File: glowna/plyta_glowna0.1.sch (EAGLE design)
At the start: 217 parts, among them IC1 4504D, IC2 MAX481CSA, IC3 4504D, IC4 OPA4658UU, Q1 CSM-7X-DU, Q2 N-HEXFET-2D_SOT232-IRLL014N, Q3 N-HEXFET-2D_SOT232-IRLL014N, Q4 N-HEXFET-2D_SOT232-IRLL014N, Q5 N-HEXFET-2D_SOT232-IRLL014N, Q6 N-HEXFET-2D_SOT232-IRLL014N, X1 MINI-USB_SHIELD5P2-32005-601

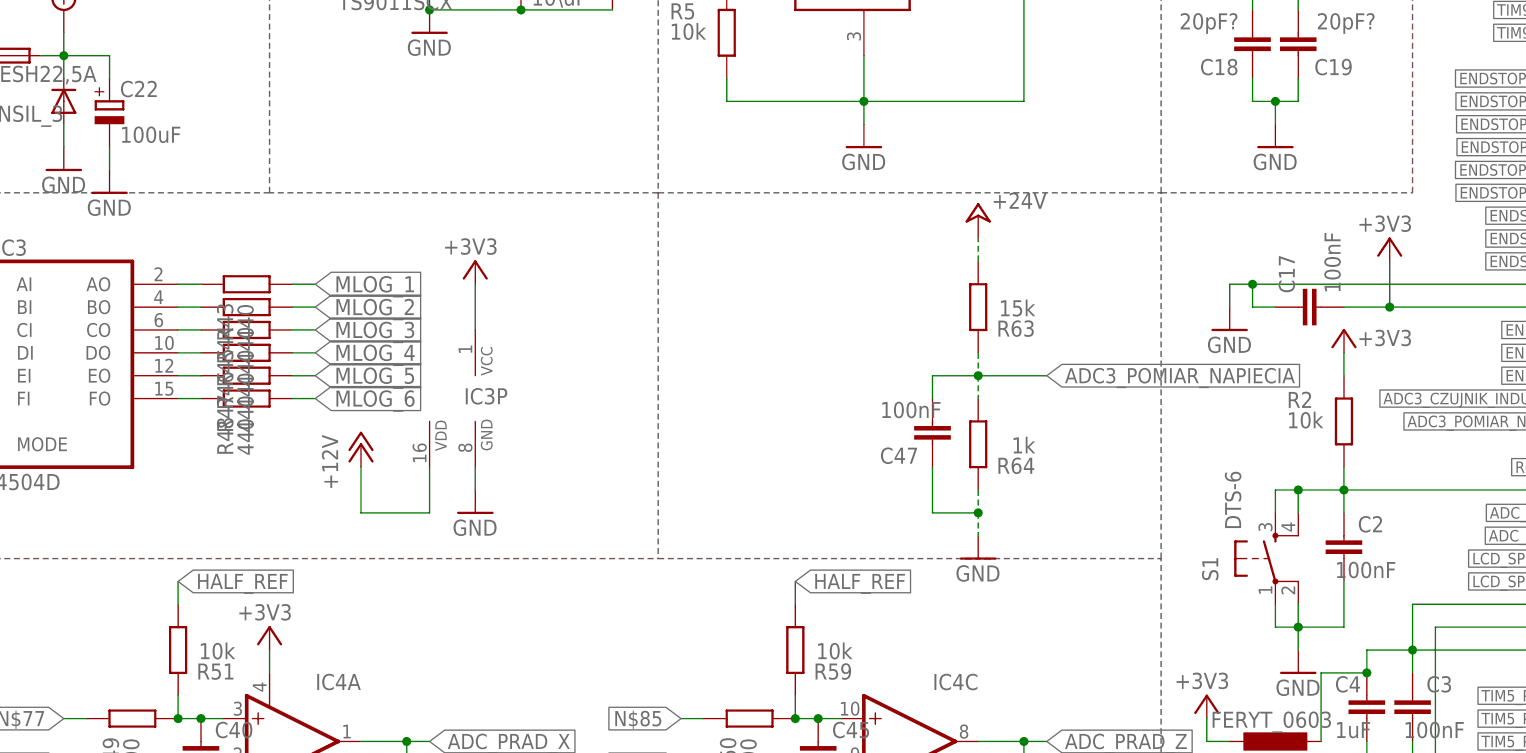
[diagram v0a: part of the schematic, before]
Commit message: zmiana
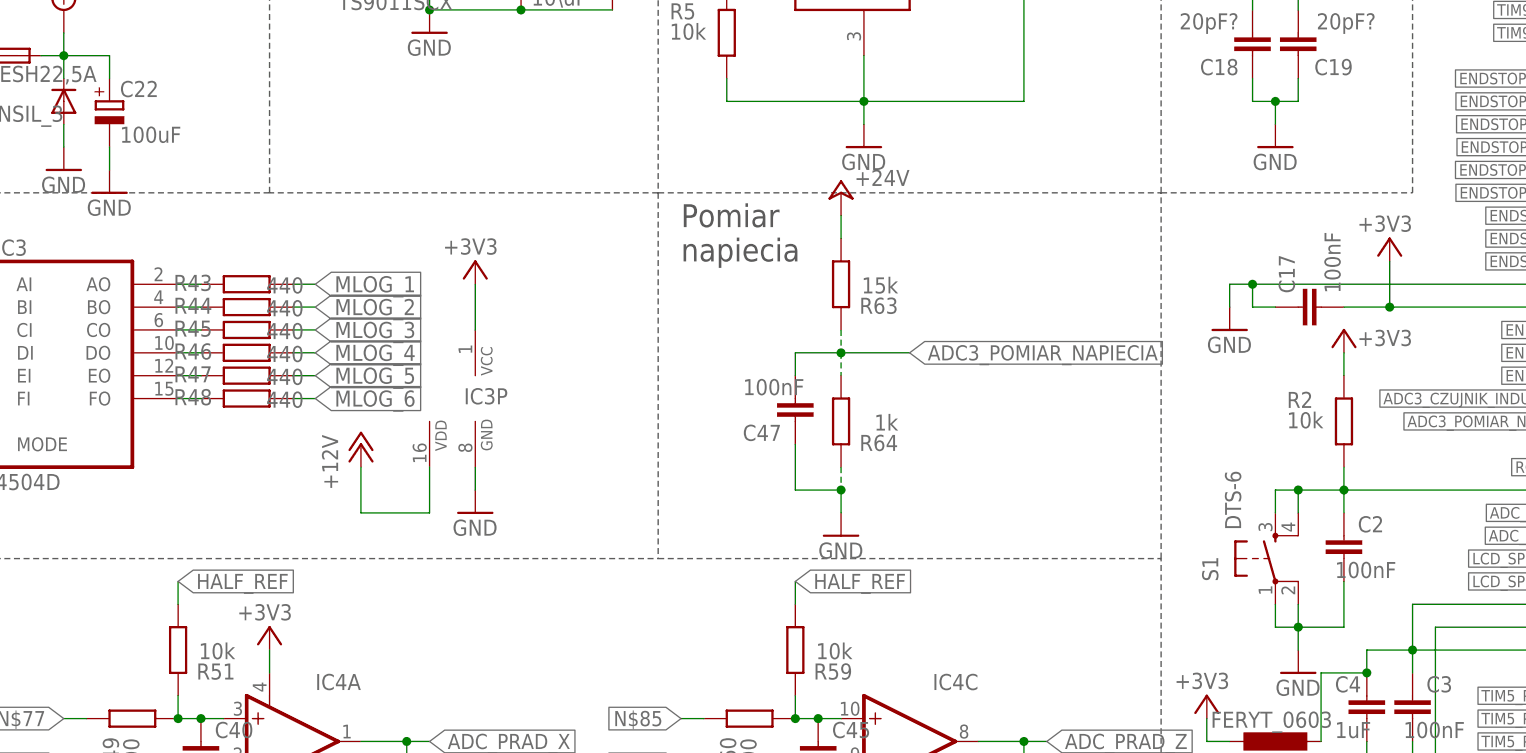
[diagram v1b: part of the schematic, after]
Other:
- note added: "Pomiar napiecia"
- moved on the sheet: C47, R63, R64
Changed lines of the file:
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@@
 <wire x1="-104.14" y1="20.32" x2="-48.26" y2="20.32" width="0.1524" layer="97" style="longdash"/>
 <wire x1="-104.14" y1="60.96" x2="-104.14" y2="20.32" width="0.1524" layer="97" style="shortdash"/>
+<text x="-101.6" y="53.34" size="2.54" layer="97">Pomiar
+napiecia</text>
 </plain>
 <instances>
@@
 <instance part="GND73" gate="1" x="-124.46" y="25.4"/>
 <instance part="R43" gate="G$1" x="-149.86" y="50.8" smashed="yes">
-<attribute name="NAME" x="-151.3586" y="44.45" size="1.778" layer="95" rot="R90"/>
-<attribute name="VALUE" x="-149.098" y="44.45" size="1.778" layer="96" rot="R90"/>
+<attribute name="NAME" x="-153.67" y="51.8414" size="1.778" layer="95" rot="R180"/>
+<attribute name="VALUE" x="-143.51" y="51.562" size="1.778" layer="96" rot="R180"/>
 </instance>
 <instance part="R44" gate="G$1" x="-149.86" y="48.26" smashed="yes">
-<attribute name="NAME" x="-151.3586" y="41.91" size="1.778" layer="95" rot="R90"/>
-<attribute name="VALUE" x="-149.098" y="41.91" size="1.778" layer="96" rot="R90"/>
+<attribute name="NAME" x="-153.67" y="49.3014" size="1.778" layer="95" rot="R180"/>
+<attribute name="VALUE" x="-143.51" y="49.022" size="1.778" layer="96" rot="R180"/>
 </instance>
 <instance part="R45" gate="G$1" x="-149.86" y="45.72" smashed="yes">
-<attribute name="NAME" x="-151.3586" y="39.37" size="1.778" layer="95" rot="R90"/>
-<attribute name="VALUE" x="-149.098" y="39.37" size="1.778" layer="96" rot="R90"/>
+<attribute name="NAME" x="-153.67" y="46.7614" size="1.778" layer="95" rot="R180"/>
+<attribute name="VALUE" x="-143.51" y="46.482" size="1.778" layer="96" rot="R180"/>
 </instance>
 <instance part="R46" gate="G$1" x="-149.86" y="43.18" smashed="yes">
-<attribute name="NAME" x="-151.3586" y="36.83" size="1.778" layer="95" rot="R90"/>
-<attribute name="VALUE" x="-149.098" y="36.83" size="1.778" layer="96" rot="R90"/>
+<attribute name="NAME" x="-153.67" y="44.2214" size="1.778" layer="95" rot="R180"/>
+<attribute name="VALUE" x="-143.51" y="43.942" size="1.778" layer="96" rot="R180"/>
 </instance>
 <instance part="R47" gate="G$1" x="-149.86" y="40.64" smashed="yes">
-<attribute name="NAME" x="-151.3586" y="34.29" size="1.778" layer="95" rot="R90"/>
-<attribute name="VALUE" x="-149.098" y="34.29" size="1.778" layer="96" rot="R90"/>
+<attribute name="NAME" x="-153.67" y="41.6814" size="1.778" layer="95" rot="R180"/>
+<attribute name="VALUE" x="-143.51" y="41.402" size="1.778" layer="96" rot="R180"/>
 </instance>
 <instance part="R48" gate="G$1" x="-149.86" y="38.1" smashed="yes">
-<attribute name="NAME" x="-151.3586" y="31.75" size="1.778" layer="95" rot="R90"/>
-<attribute name="VALUE" x="-149.098" y="31.75" size="1.778" layer="96" rot="R90"/>
+<attribute name="NAME" x="-153.67" y="39.1414" size="1.778" layer="95" rot="R180"/>
+<attribute name="VALUE" x="-143.51" y="38.862" size="1.778" layer="96" rot="R180"/>
 </instance>
 <instance part="GND74" gate="1" x="-185.42" y="25.4"/>
@@
 <attribute name="VALUE" x="-67.564" y="-15.621" size="1.778" layer="96" rot="R180"/>
 </instance>
-<instance part="R63" gate="G$1" x="-68.58" y="48.26" smashed="yes" rot="R90">
-<attribute name="NAME" x="-62.23" y="46.7614" size="1.778" layer="95" rot="R180"/>
-<attribute name="VALUE" x="-62.23" y="49.022" size="1.778" layer="96" rot="R180"/>
-</instance>
-<instance part="R64" gate="G$1" x="-68.58" y="33.02" smashed="yes" rot="R90">
-<attribute name="NAME" x="-62.23" y="31.5214" size="1.778" layer="95" rot="R180"/>
-<attribute name="VALUE" x="-62.23" y="33.782" size="1.778" layer="96" rot="R180"/>
-</instance>
-<instance part="GND77" gate="1" x="-68.58" y="20.32"/>
-<instance part="P+10" gate="1" x="-68.58" y="58.42" smashed="yes">
-<attribute name="VALUE" x="-60.96" y="60.96" size="1.778" layer="96" rot="R180"/>
-</instance>
-<instance part="C47" gate="G$1" x="-73.66" y="33.02" smashed="yes" rot="R180">
-<attribute name="NAME" x="-75.184" y="32.639" size="1.778" layer="95" rot="R180"/>
-<attribute name="VALUE" x="-72.644" y="37.719" size="1.778" layer="96" rot="R180"/>
+<instance part="R63" gate="G$1" x="-83.82" y="50.8" smashed="yes" rot="R90">
+<attribute name="NAME" x="-77.47" y="49.3014" size="1.778" layer="95" rot="R180"/>
+<attribute name="VALUE" x="-77.47" y="51.562" size="1.778" layer="96" rot="R180"/>
+</instance>
+<instance part="R64" gate="G$1" x="-83.82" y="35.56" smashed="yes" rot="R90">
+<attribute name="NAME" x="-77.47" y="34.0614" size="1.778" layer="95" rot="R180"/>
+<attribute name="VALUE" x="-77.47" y="36.322" size="1.778" layer="96" rot="R180"/>
+</instance>
+<instance part="GND77" gate="1" x="-83.82" y="22.86"/>
+<instance part="P+10" gate="1" x="-83.82" y="60.96" smashed="yes">
+<attribute name="VALUE" x="-76.2" y="63.5" size="1.778" layer="96" rot="R180"/>
+</instance>
+<instance part="C47" gate="G$1" x="-88.9" y="35.56" smashed="yes" rot="R180">
+<attribute name="NAME" x="-90.424" y="35.179" size="1.778" layer="95" rot="R180"/>
+<attribute name="VALUE" x="-87.884" y="40.259" size="1.778" layer="96" rot="R180"/>
 </instance>
 <instance part="JP23" gate="G$1" x="231.14" y="12.7"/>
@@
 </segment>
 <segment>
-<pinref part="R64" gate="G$1" pin="1"/>
-<wire x1="-68.58" y1="27.94" x2="-68.58" y2="25.4" width="0.1524" layer="91" style="longdash"/>
-<pinref part="GND77" gate="1" pin="GND"/>
-<pinref part="C47" gate="G$1" pin="1"/>
-<wire x1="-68.58" y1="25.4" x2="-68.58" y2="22.86" width="0.1524" layer="91" style="longdash"/>
-<wire x1="-68.58" y1="25.4" x2="-73.66" y2="25.4" width="0.1524" layer="91"/>
-<wire x1="-73.66" y1="25.4" x2="-73.66" y2="30.48" width="0.1524" layer="91"/>
-<junction x="-68.58" y="25.4"/>
-</segment>
-<segment>
 <pinref part="GND76" gate="1" pin="GND"/>
 <pinref part="R53" gate="G$1" pin="1"/>
@@
 <junction x="-91.44" y="-43.18"/>
 </segment>
+<segment>
+<pinref part="R64" gate="G$1" pin="1"/>
+<wire x1="-83.82" y1="30.48" x2="-83.82" y2="27.94" width="0.1524" layer="91" style="longdash"/>
+<pinref part="C47" gate="G$1" pin="1"/>
+<wire x1="-83.82" y1="27.94" x2="-88.9" y2="27.94" width="0.1524" layer="91"/>
+<wire x1="-88.9" y1="27.94" x2="-88.9" y2="33.02" width="0.1524" layer="91"/>
+<pinref part="GND77" gate="1" pin="GND"/>
+<wire x1="-83.82" y1="25.4" x2="-83.82" y2="27.94" width="0.1524" layer="91"/>
+<junction x="-83.82" y="27.94"/>
+</segment>
 </net>
 <net name="I2C1_SDA" class="0">
@@
 <pinref part="R63" gate="G$1" pin="1"/>
 <pinref part="R64" gate="G$1" pin="2"/>
-<wire x1="-68.58" y1="43.18" x2="-68.58" y2="40.64" width="0.1524" layer="91" style="longdash"/>
-<wire x1="-68.58" y1="40.64" x2="-68.58" y2="38.1" width="0.1524" layer="91" style="longdash"/>
-<wire x1="-68.58" y1="40.64" x2="-60.96" y2="40.64" width="0.1524" layer="91"/>
-<junction x="-68.58" y="40.64"/>
-<label x="-60.96" y="40.64" size="1.6764" layer="95" xref="yes"/>
+<wire x1="-83.82" y1="45.72" x2="-83.82" y2="43.18" width="0.1524" layer="91" style="longdash"/>
+<wire x1="-83.82" y1="43.18" x2="-83.82" y2="40.64" width="0.1524" layer="91" style="longdash"/>
+<wire x1="-83.82" y1="43.18" x2="-76.2" y2="43.18" width="0.1524" layer="91"/>
+<junction x="-83.82" y="43.18"/>
+<label x="-76.2" y="43.18" size="1.6764" layer="95" xref="yes"/>
 <pinref part="C47" gate="G$1" pin="2"/>
-<wire x1="-68.58" y1="40.64" x2="-73.66" y2="40.64" width="0.1524" layer="91"/>
-<wire x1="-73.66" y1="40.64" x2="-73.66" y2="38.1" width="0.1524" layer="91"/>
+<wire x1="-83.82" y1="43.18" x2="-88.9" y2="43.18" width="0.1524" layer="91"/>
+<wire x1="-88.9" y1="43.18" x2="-88.9" y2="40.64" width="0.1524" layer="91"/>
 </segment>
 </net>
@@
 <segment>
 <pinref part="R63" gate="G$1" pin="2"/>
-<wire x1="-68.58" y1="53.34" x2="-68.58" y2="55.88" width="0.1524" layer="91" style="longdash"/>
 <pinref part="P+10" gate="1" pin="+24V"/>
+<wire x1="-83.82" y1="58.42" x2="-83.82" y2="55.88" width="0.1524" layer="91"/>
 </segment>
 </net>
